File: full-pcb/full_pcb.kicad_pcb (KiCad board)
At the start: 4 copper layers, 73.5 x 129.7 mm, 51 parts, among them J1 Screw_Terminal_01x02, J3 Barrel_Jack_Switch, J4 AUDIO_IN_TRS, J5 AUDIO_OUT_TRS, J6 Screw_Terminal_01x02, J7 AUDIO_IN_TRS, J8 AUDIO_OUT_TRS, U1 78L05G-AB3-R, U2 OPA1664D, U3 TPS5430DDA, U4 CJ431, U5 XIAO-ESP32-C6-DIP (2 1x7 pin 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

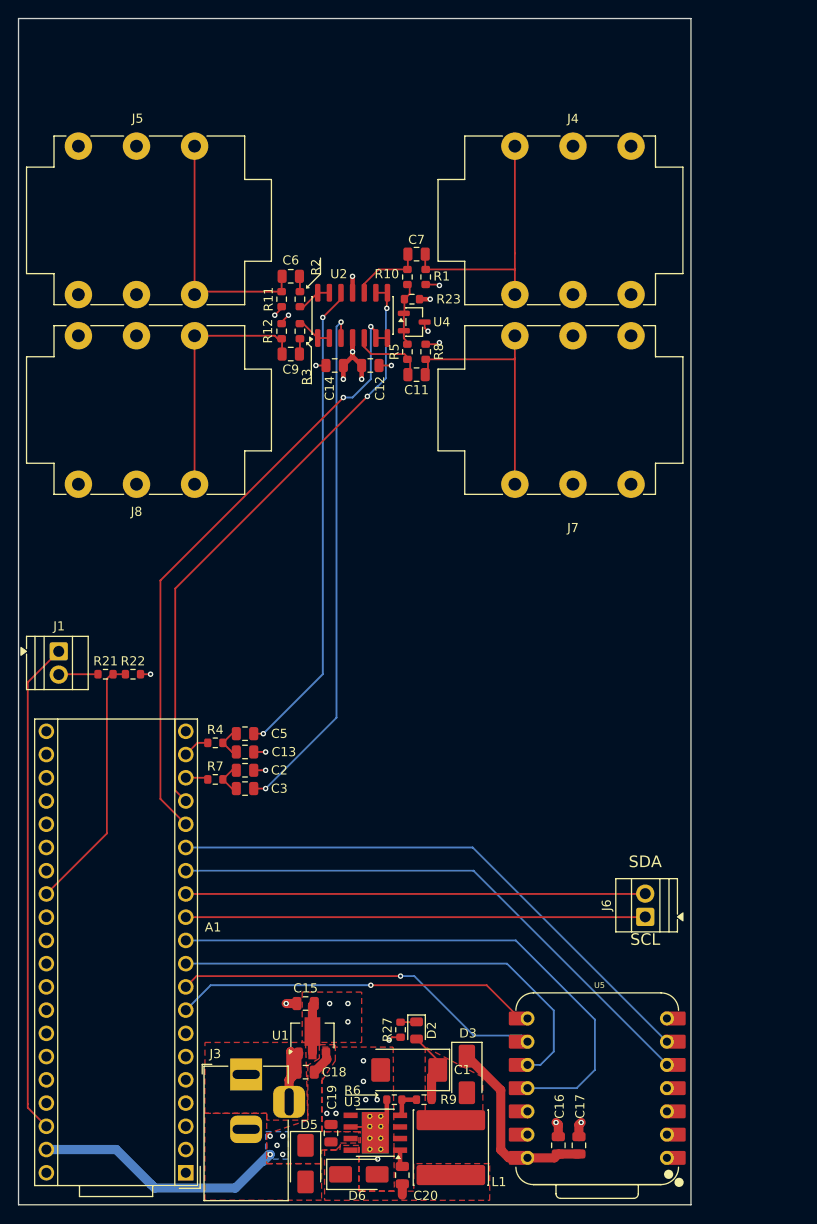
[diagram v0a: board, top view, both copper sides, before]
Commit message: pedal works but is buggy
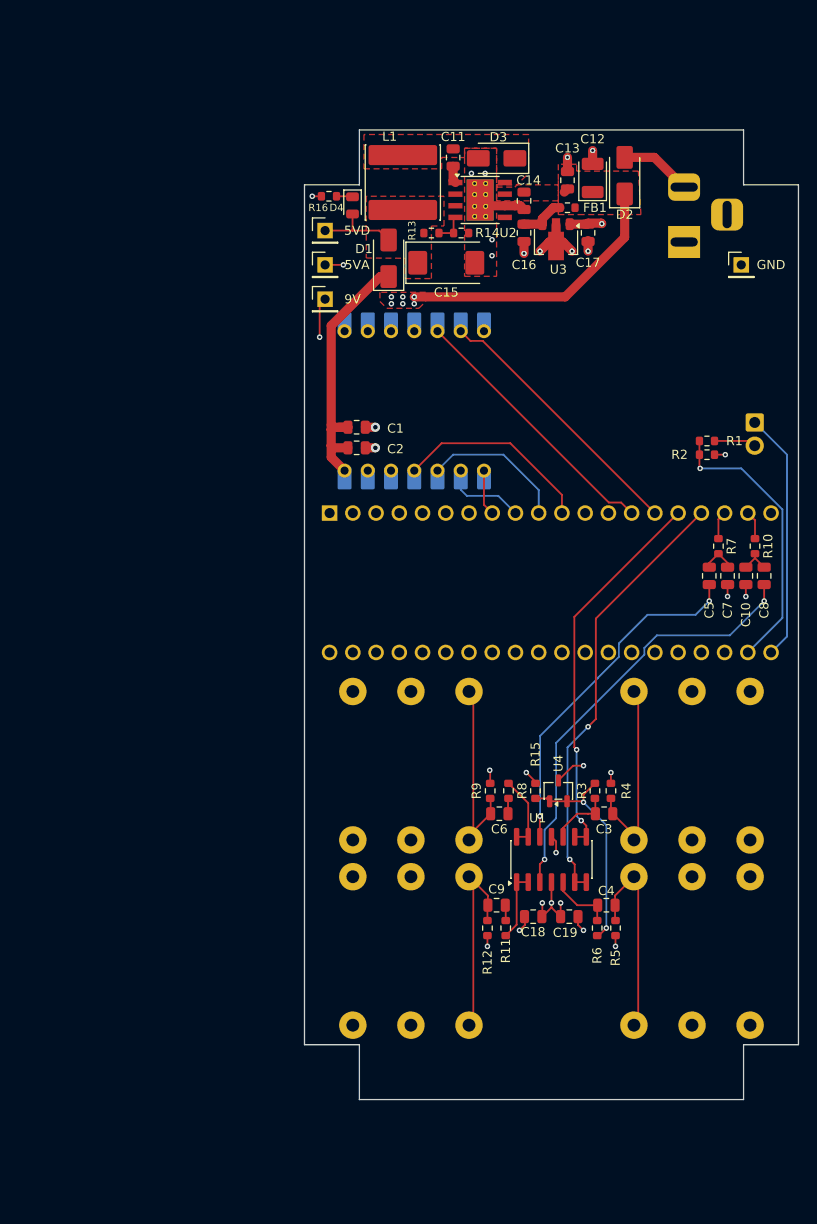
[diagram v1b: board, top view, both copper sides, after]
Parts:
- removed the C15 at (150.6, 139.2)
- removed the J1 at (123.6, 100.8)
- removed the J6 at (187.8, 129.8)
- removed R21: 100, Resistor_SMD:R_0603_1608Metric
- removed R22: 10k, Resistor_SMD:R_0603_1608Metric
- removed R27: 1K, Resistor_SMD:R_0603_1608Metric
- added 5VA1: TestPoint, Connector_PinHeader_2.54mm:PinHeader_1x01_P2.54mm_Vertical, F.Cu at (152.8, 58.5)
- added 5VD1: TestPoint, Connector_PinHeader_2.54mm:PinHeader_1x01_P2.54mm_Vertical, F.Cu at (152.8, 54.8)
- added 9V1: TestPoint, Connector_PinHeader_2.54mm:PinHeader_1x01_P2.54mm_Vertical, F.Cu at (152.8, 62.2)
- added C12: 100uf, Capacitor_Tantalum_SMD:CP_EIA-3528-21_Kemet-B, F.Cu at (182.0, 49.0)
- added C16: 0.33uf, Capacitor_SMD:C_0805_2012Metric, F.Cu at (174.5, 55.0)
- added C17: 0.1uf, Capacitor_SMD:C_0805_2012Metric, F.Cu at (181.5, 55.0)
- added FB1: 120Ω@100MHz, Resistor_SMD:R_0603_1608Metric, F.Cu at (179.2, 52.2)
- added GND1: TestPoint, Connector_PinHeader_2.54mm:PinHeader_1x01_P2.54mm_Vertical, F.Cu at (198.2, 58.5)
- added J3: Screw_Terminal_01x02, TerminalBlock:TerminalBlock_Xinya_XY308-2.54-2P_1x02_P2.54mm_Horizontal, B.Cu at (199.7, 75.7)
- added R1: 100, Resistor_SMD:R_0603_1608Metric, F.Cu at (194.5, 77.8)
- added R16: 10k, Resistor_SMD:R_0603_1608Metric, F.Cu at (153.2, 51.0)
- added R2: 10k, Resistor_SMD:R_0603_1608Metric, F.Cu at (194.5, 79.2)
- A1, J4, J5: moved to B.Cu
- A2: renamed from U5; moved to B.Cu
- C18: value 10uf -> 0.1uf
- J1: renamed from J7; moved to B.Cu
- J2: renamed from J8; moved to B.Cu
- J6: renamed from J3; moved to B.Cu
- R14: renamed from R6; value 3.24k -> 3.3k
- moved D2 113.5 mm to (185.5, 48.8), turned to 90 degrees
- moved D3 112.1 mm to (171.5, 46.9), turned to 180 degrees
- moved C11 111.4 mm to (166.8, 46.8), turned to 90 degrees
- moved C13 107.3 mm to (179.2, 49.2)
- moved L1 105.6 mm to (161.2, 49.5), turned to -90 degrees
- moved J6 102.8 mm to (192.0, 56.0), turned to -90 degrees
- moved U2 102.6 mm to (169.7, 51.4), turned to 0 degrees
- moved J4 97.0 mm to (186.5, 141.6)
- moved R14 95.0 mm to (167.6, 55.0), turned to 0 degrees
- moved R13 94.7 mm to (164.4, 55.0), turned to 0 degrees
- moved U3 90.7 mm to (178.0, 56.0), turned to -90 degrees
- moved D4 90.5 mm to (155.8, 52.0)
- moved D1 89.6 mm to (159.7, 57.8), turned to 90 degrees
- moved C15 88.3 mm to (166.0, 58.3), turned to 0 degrees
- moved C1 81.5 mm to (156.2, 76.2), turned to 0 degrees
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- renumbered C16 to C1, C13 to C10, C20 to C11, C19 to C13, C1 to C15, C12 to C19, C17 to C2, C11 to C3, C7 to C4, C3 to C5, C9 to C6, C2 to C7, C5 to C8, C6 to C9, D3 to D1, D5 to D2, D6 to D3, D2 to D4, R4 to R10, R2 to R11, R11 to R12, R9 to R13, R23 to R15, R5 to R3, R8 to R4, R1 to R5, R10 to R6, R3 to R8, R12 to R9, U2 to U1, U3 to U2, U1 to U3
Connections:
- A1 pad 12: Net-(A1-I2C1_SCL) -> unconnected-(A1-I2C1_SCL-Pad12)
- A1 pad 13: Net-(A1-I2C1_SDA) -> unconnected-(A1-I2C1_SDA-Pad13)
- A1 pad 22: unconnected-(A1-ADC_0-Pad22) -> Net-(A1-ADC_0)
- A1 pad 28: Net-(A1-ADC_6) -> unconnected-(A1-ADC_6-Pad28)
- C14 pad 1: +5VA -> GND
- C14 pad 2: GND -> +9V
- C18 pad 1: GND -> +5VA
- C18 pad 2: +9V -> GND
- C3 pad 2: Net-(U2B-+) -> Net-(U1C-+)
- C4 pad 2: Net-(U2C-+) -> Net-(U1B-+)
- C5 pad 2: Net-(U2A-+) -> Net-(U1D-+)
- C8 pad 2: Net-(U2D-+) -> Net-(U1A-+)
- R11 pad 1: Net-(U2D--) -> Net-(U1A--)
- R3 pad 1: Net-(U2B-+) -> Net-(U1C-+)
- R5 pad 1: Net-(U2C-+) -> Net-(U1B-+)
- R8 pad 1: Net-(U2A--) -> Net-(U1D--)
- U1 pad 1: Net-(U2A--) -> Net-(U1A--)
- U1 pad 10: Net-(U2C-+) -> Net-(U1C-+)
- U1 pad 12: Net-(U2D-+) -> Net-(U1D-+)
- U1 pad 13: Net-(U2D--) -> Net-(U1D--)
- U1 pad 14: Net-(U2D--) -> Net-(U1D--)
- U1 pad 2: Net-(U2A--) -> Net-(U1A--)
- U1 pad 3: Net-(U2A-+) -> Net-(U1A-+)
- U1 pad 5: Net-(U2B-+) -> Net-(U1B-+)
- U1 pad 6: AUDIO_IN_JACK_RIGHT_BUF -> AUDIO_IN_JACK_LEFT_BUF
- U1 pad 7: AUDIO_IN_JACK_RIGHT_BUF -> AUDIO_IN_JACK_LEFT_BUF
- U1 pad 8: AUDIO_IN_JACK_LEFT_BUF -> AUDIO_IN_JACK_RIGHT_BUF
- U1 pad 9: AUDIO_IN_JACK_LEFT_BUF -> AUDIO_IN_JACK_RIGHT_BUF
- U3 pad 1: GND -> +5VA
- U3 pad 2: +5VA -> GND
- U3 pad 3: +9V -> Net-(U3-VI)
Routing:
- net Net-(U2A-+): track 57.5 -> 0.00 mm, vias 2 -> 0
- net +3.3VD: track 54.2 -> 0.00 mm
- net Net-(U2D-+): track 52.8 -> 0.00 mm, vias 2 -> 0
- net Net-(A1-I2C1_SCL): track 50.4 -> 0.00 mm
- net Net-(A1-I2C1_SDA): track 50.4 -> 0.00 mm
- net +9V: track 31.2 -> 80.6 mm, vias 5 -> 7
- net Net-(U1A-+): track 0.00 -> 47.4 mm, vias 0 -> 2
- net PICO: track 63.1 -> 21.7 mm
- net Net-(U1D-+): track 0.00 -> 38.3 mm, vias 0 -> 2
- net CS: track 39.2 -> 5.01 mm, vias 1 -> 0
- net POCI: track 50.6 -> 16.8 mm
- net SCK: track 41.8 -> 8.29 mm, vias 1 -> 0
- net DAISY_OUT: track 62.4 -> 29.5 mm
- net DAISY_IN: track 61.4 -> 29.5 mm
- net Net-(A1-ADC_0): track 0.00 -> 31.1 mm, vias 0 -> 1
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- added copper zone on In2.Cu, net +9V
- removed copper zone on F.Cu, net +5VA
- removed copper zone on B.Cu, net +9V
- removed copper zone on F.Cu, net POWER_JACK_PWR
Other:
- board size 73.5 x 129.7 mm -> 54 x 106 mm
- board text added: "5VA"
- board text added: "5VD"
- board text added: "9V"
- board text added: "GND"
- board text removed: "SCL"
- board text removed: "SDA"
